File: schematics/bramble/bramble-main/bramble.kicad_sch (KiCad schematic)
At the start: 13 parts, among them U1 Opamp_Quad

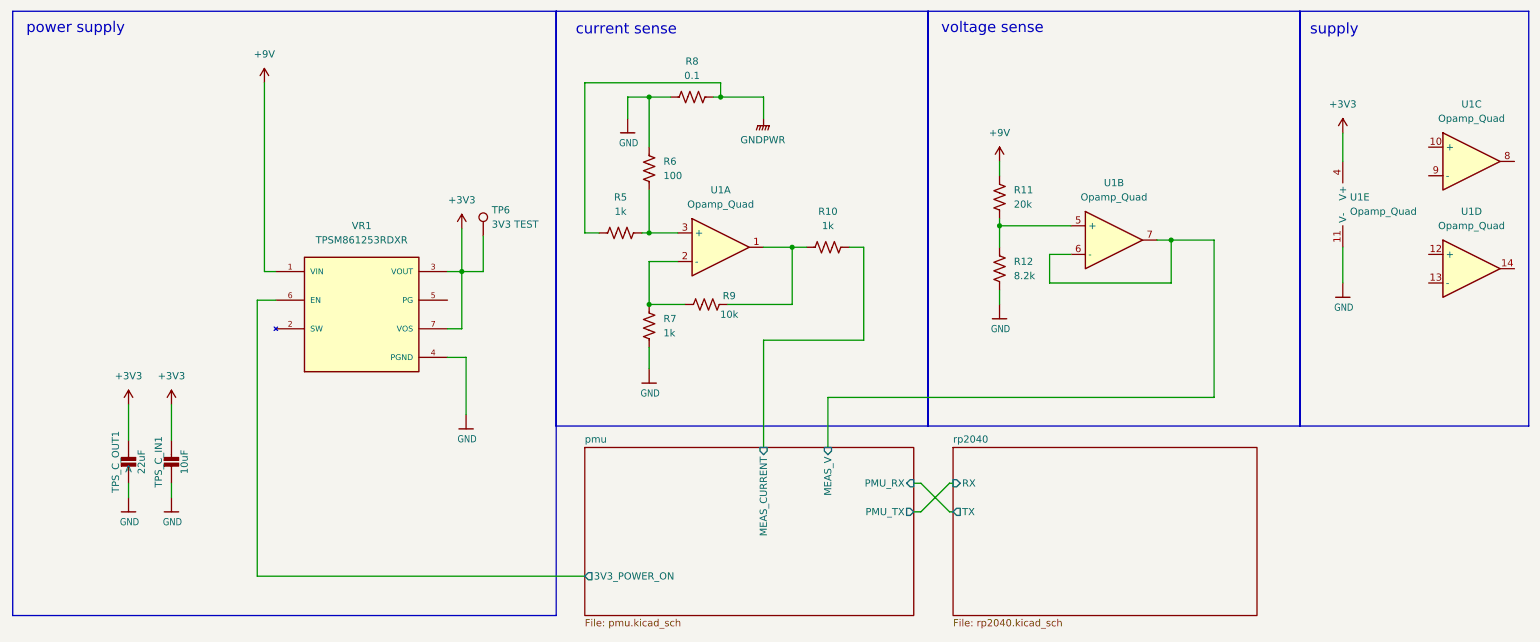
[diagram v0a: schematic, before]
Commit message: Checking in v4 schematic/board prior to attempting jlcpcb run
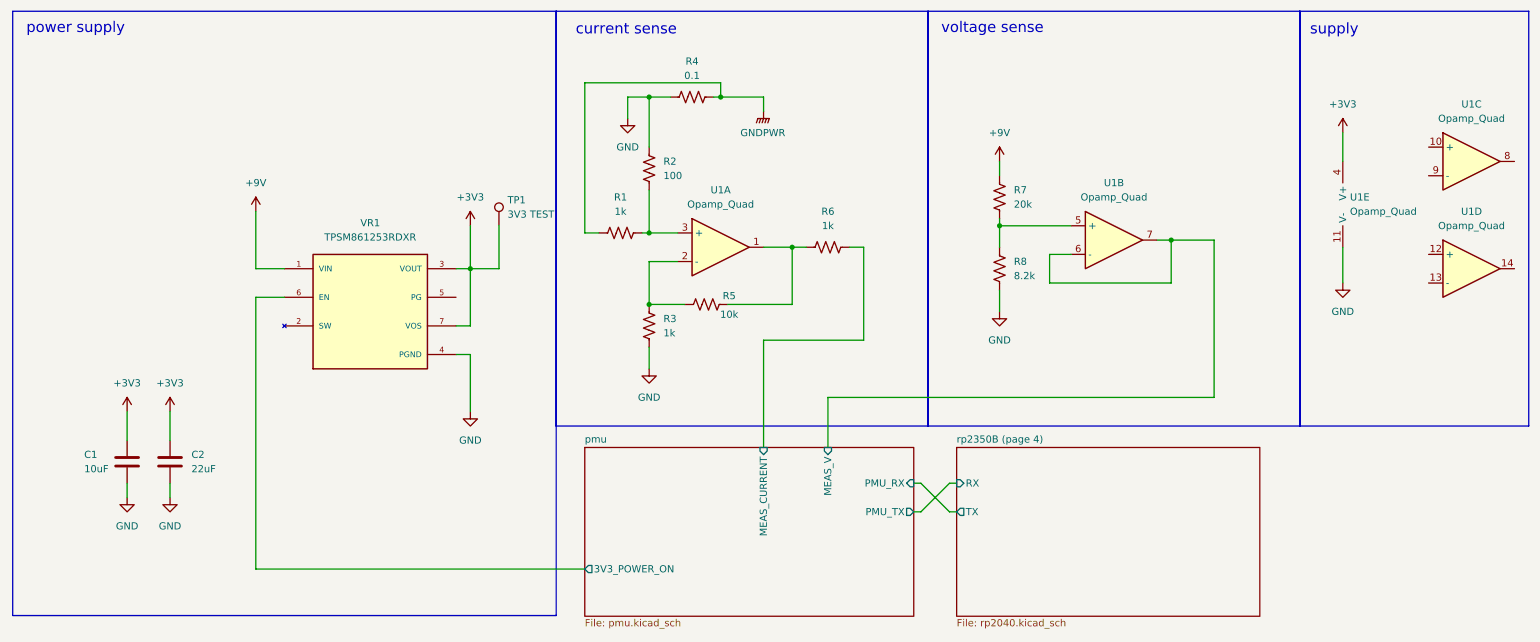
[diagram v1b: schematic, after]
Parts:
- removed TPS_C_IN1: 10uF, Capacitor_SMD:C_0805_2012Metric, symbol Adafruit Feather RP2040 RFM-eagle-import:CAP_CERAMIC0805-NOOUTLINE
- removed TPS_C_OUT1: 22uF, Capacitor_SMD:C_0805_2012Metric, symbol Adafruit Feather RP2040 RFM-eagle-import:CAP_CERAMIC0805-NOOUTLINE
- added C1: 10uF, Capacitor_SMD:C_0805_2012Metric, symbol Device:C
- added C2: 22uF, Capacitor_SMD:C_0805_2012Metric, symbol Device:C
- renumbered R5 to R1, R6 to R2, R7 to R3, R8 to R4, R9 to R5, R10 to R6, R11 to R7, R12 to R8, TP6 to TP1
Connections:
- net +3V3: now also C1.1, C2.1
- net GND: now also C1.2, C2.2
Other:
- sheet rp2040 renamed rp2350B (page 4)
- moved on the sheet: TP1, VR1
